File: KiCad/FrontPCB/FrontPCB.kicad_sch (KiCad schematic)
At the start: 18 parts, among them U1 ESP32-S3-WROOM-1

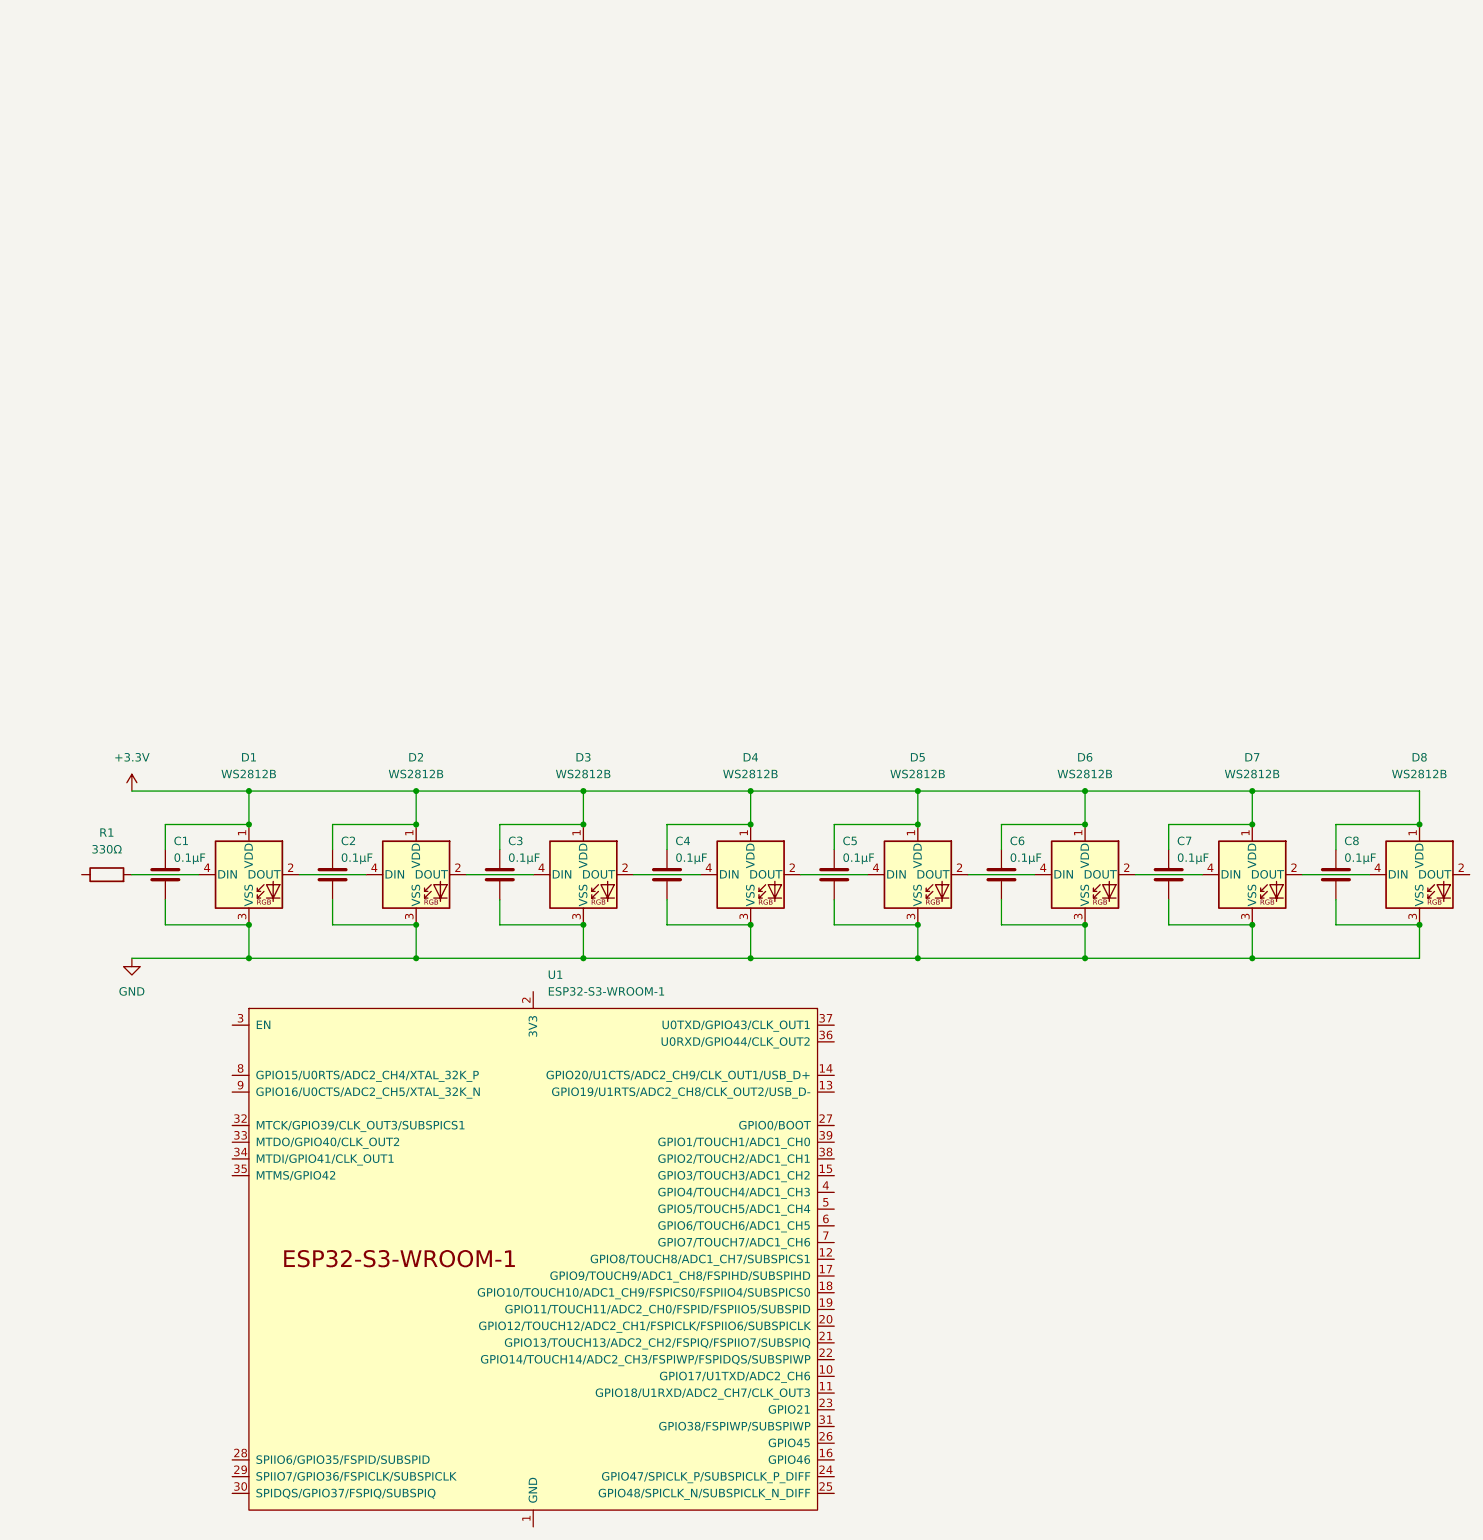
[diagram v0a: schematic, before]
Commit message: CHG: changed wiring of front PCB
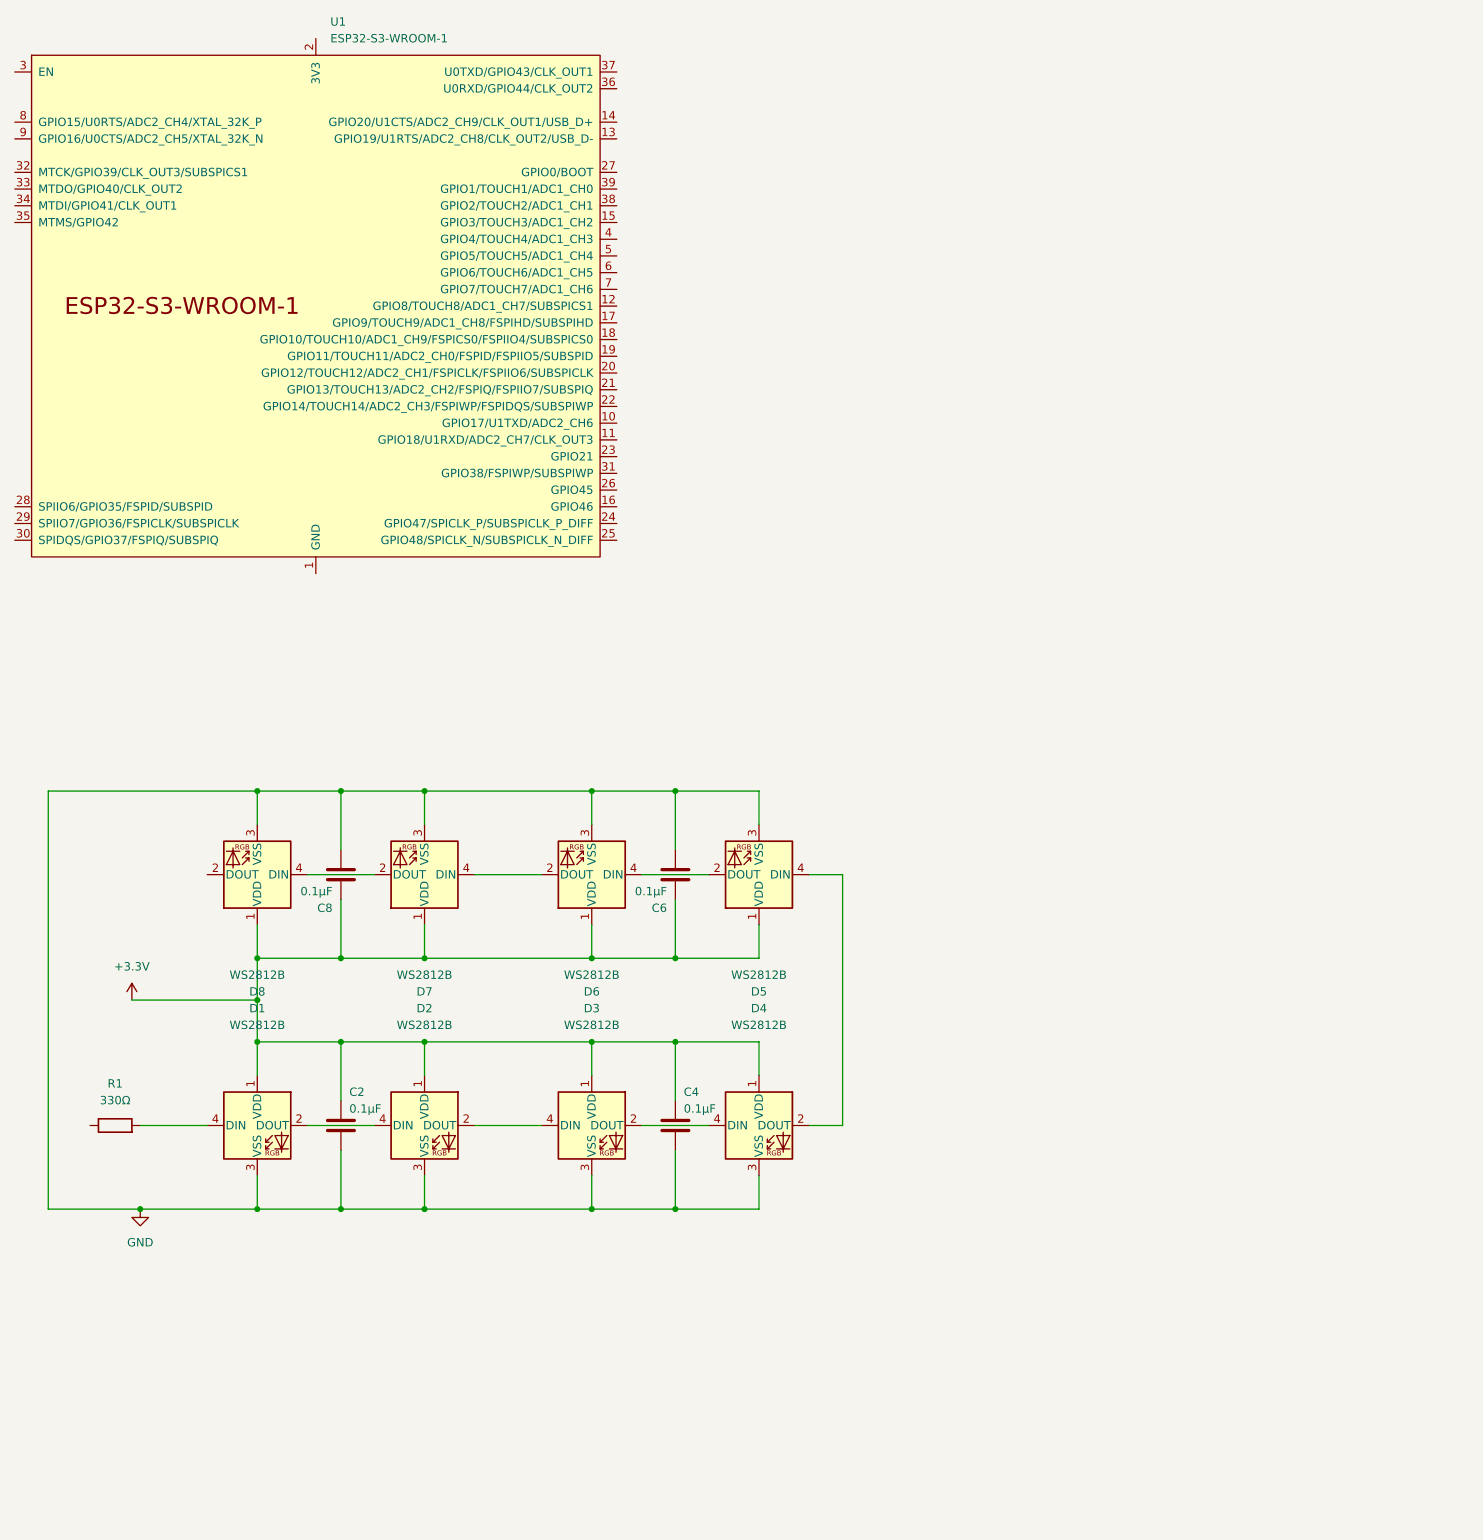
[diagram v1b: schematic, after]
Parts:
- removed C1, C3, C5, C7: 0.1µF, Capacitor_SMD:C_0805_2012Metric, symbol Device:C
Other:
- moved on the sheet: C2, C4, C6, C8, D1, D2, D3, D4, D5, D6, D7, D8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
